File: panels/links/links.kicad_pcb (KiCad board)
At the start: 2 copper layers, 20 x 128.5 mm, 0 parts

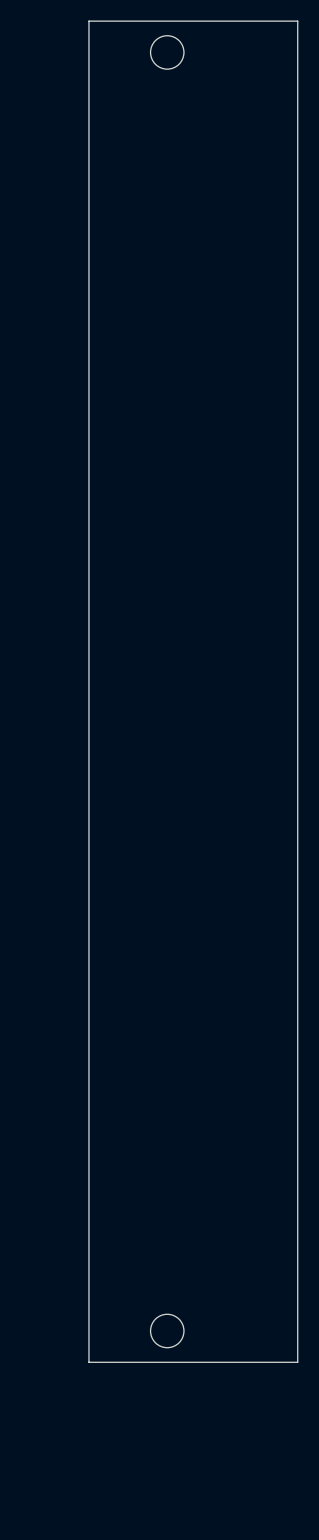
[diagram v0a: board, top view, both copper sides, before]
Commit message: Links Panel Desgin
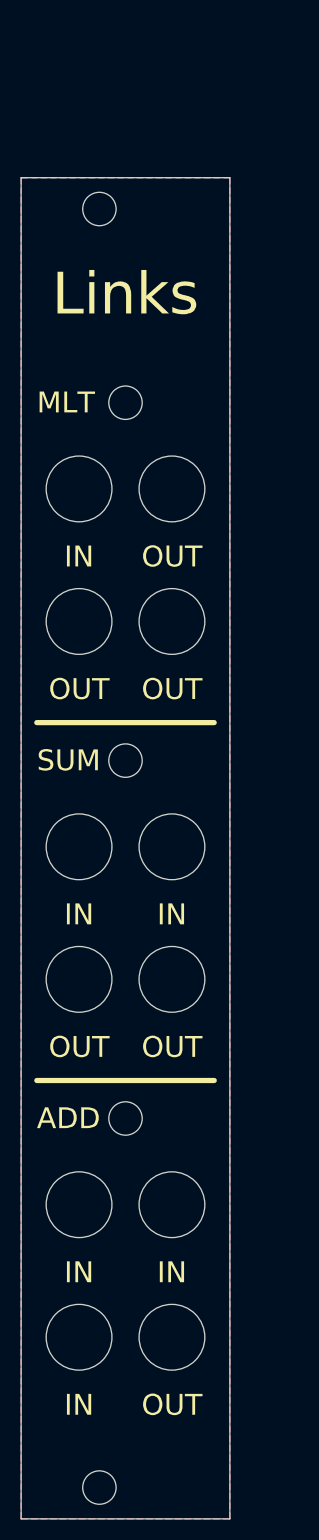
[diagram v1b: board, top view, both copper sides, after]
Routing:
- added copper zone on B.Cu, net (none)
- added copper zone on F.Cu, net (none)
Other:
- outline, holes or cut-outs redrawn
- board text added: "ADD"
- board text added: "IN"
- board text added: "Links"
- board text added: "MLT"
- board text added: "OUT"
- board text added: "SUM"
- board text added: "www.birchavenue.org"
